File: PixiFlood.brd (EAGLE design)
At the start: 43.2 x 46 mm, 36 parts, among them IC1 WS2811-SOP8, IC2 78L05Z, T1 2N3904, T2 2N3904, T3 2N3904, U1 PT4115B89E, U2 PT4115B89E, U3 PT4115B89E, X2 22-23-2041

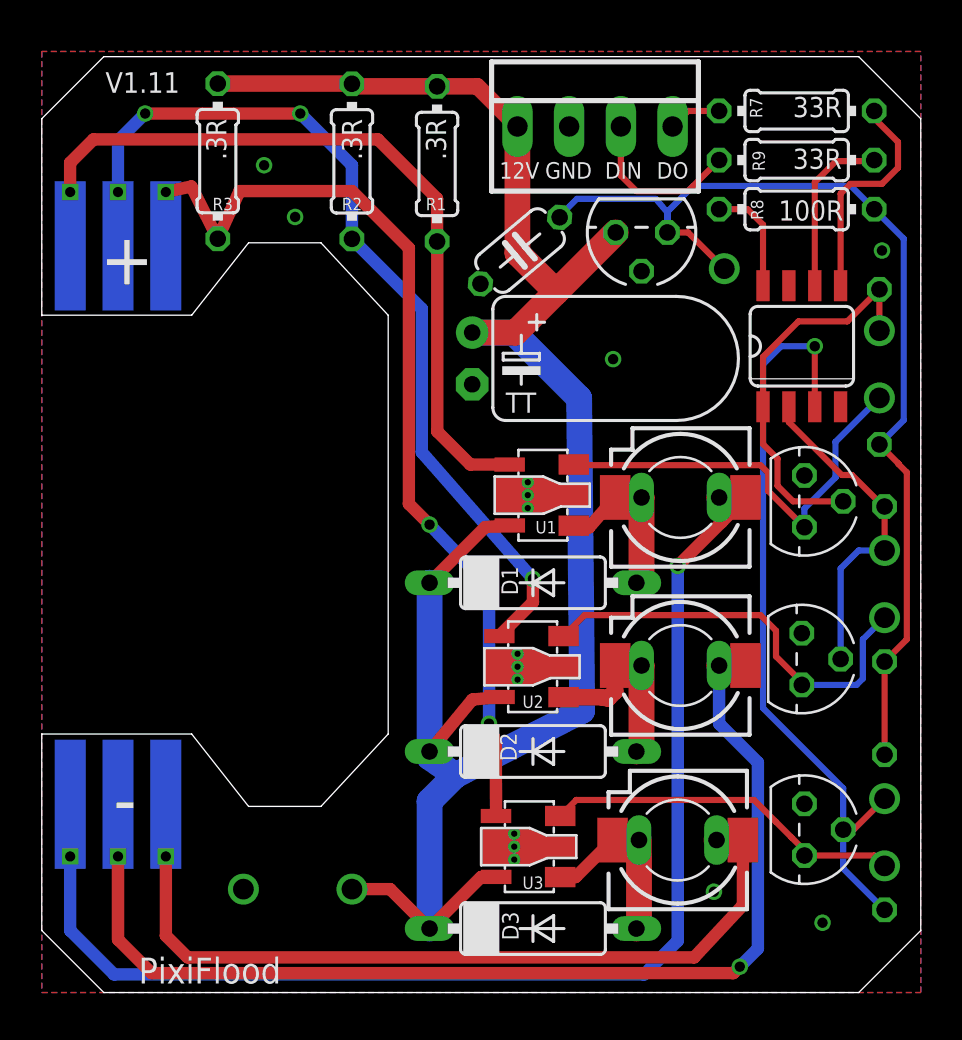
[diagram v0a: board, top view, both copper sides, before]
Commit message: Initial Commit
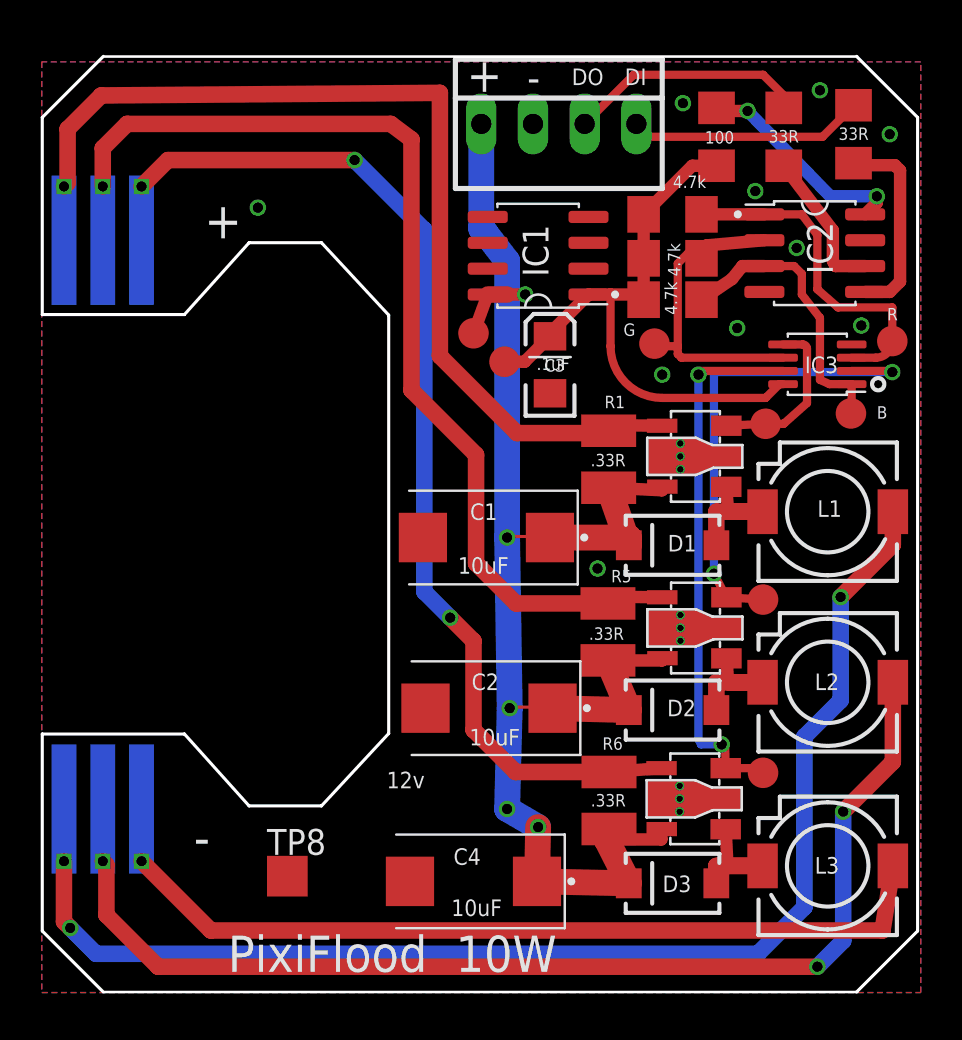
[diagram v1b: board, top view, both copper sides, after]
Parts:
- removed T$1, T$2, T$3, T$4, T$5, T$6, T$7, T$8, T$9: TEST_PINTP-2, headers:TP-2
- removed T1, T2, T3: 2N3904, transistor:TO92
- removed X2: 22-23-2041, connectors:22-23-2041
- added C3: .1uF, capacitors:EIA3216
- added C4: 10uF, capacitors:VISHAY-CASE-D
- added IC3: TC7W04FP-0.65, logic:SSOP8-0.65P-(TSSOP8)
- added TP1, TP2, TP3, TP4, TP5, TP6, TP7, TP9: TPSQTP15R, testpad:TP15R
- added TP8: TPSQTP20SQ, testpad:TP20SQ
- added X1: 22-23-2041, connectors:22-23-2041
- B1: value LED-BOARDNODIM -> LED-BOARDV4; device myBoards:LED_BOARD_V5_A -> special:LED_BOARD-V4
- C1: value 100uF -> 10uF; device rcl:TT2D6L -> capacitors:VISHAY-CASE-D
- C2: value .1uF -> 10uF; device rcl:C050-024X044 -> capacitors:VISHAY-CASE-D
- D1, D2, D3: value 1N5819 -> B340A; device diode:DO07 -> SparkFun-DiscreteSemi:SMA-DIODE
- IC1: value WS2811-SOP8 -> 78L05SMD; device MyLibrary:SO08-SKINNYPADS -> regulators:SO08
- IC2: value 78L05Z -> WS2811S; device linear:TO92 -> drivers:SO08
- L1, L2, L3: value INDUCTOR82114R -> SLF7045T-101MR60-H; device rcl:82114R-C -> inductors:SLF7045
- R1: value .3R -> .33R; device resistor:0204/7 -> resistor:R1210
- R2, R3: value .3R -> 33R; device resistor:0204/7 -> rcl:R1206
- R4: value 4.7k -> 100; device resistor:0204/7 -> rcl:R1206
- R5, R6: value 4.7k -> .33R; device resistor:0204/7 -> resistor:R1210
- R7, R9: value 33R -> 4.7k; device rcl:0204/7 -> rcl:R1206
- R8: value 100R -> 4.7k; device rcl:0204/7 -> rcl:R1206
- moved R3 31.3 mm to (39.9, 42.2)
- moved C2 22.5 mm to (22.0, 14.0), turned to 0 degrees
- moved R2 21.2 mm to (36.4, 42.0)
- moved R1 16.8 mm to (27.8, 26.2)
- moved R4 13.8 mm to (33.1, 42.0), flipped to the top
- moved R5 13.8 mm to (27.8, 17.7), flipped to the top, turned to 270 degrees
- moved IC1 13.7 mm to (24.4, 36.2), turned to 90 degrees
- moved R6 13.6 mm to (27.9, 9.43), flipped to the top
- moved R7 11.1 mm to (31.0, 34.0)
- moved C1 8.82 mm to (21.8, 22.4), turned to 0 degrees
- moved IC2 8.57 mm to (38.0, 36.3), turned to 0 degrees
- moved U3 8.46 mm to (32.1, 9.52)
- moved U2 8.22 mm to (32.1, 17.9)
- moved U1 7.73 mm to (32.1, 26.3)
- moved L3 7.47 mm to (38.6, 6.22), turned to 0 degrees
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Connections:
- removed net +12V: C1.+, D1.C, D2.C, D3.C, IC2.3, R1.1, R2.1, R3.1, T$9.P$1, U1.5, U2.5, U3.5, X2.1
- removed net DIN-R: IC1.6, R9.2
- removed net DO-R: IC1.5, R7.2
- removed net N$15: IC1.3, R6.2, T$5.P$1, T3.2
- removed net N$18: IC1.2, R5.2, T$4.P$1, T2.2
- removed net N$20: IC1.1, R4.2, T$1.P$1, T1.2
- new net BLU-WS: IC2.3, IC3.1, R7.2, TP2.TP
- new net DIN-E: R2.1, X1.3
- new net DO-E: R3.1, X1.4
- new net GREN-WS: IC2.2, IC3.6, R8.2, TP3.TP
- new net RED-WS: IC2.1, IC3.3, R9.2, TP7.TP
- new net VIN: C1.1, C2.1, C4.1, D1.C, D2.C, D3.C, IC1.8, R1.2, R5.2, R6.2, TP4.TP, U1.5, U2.5, U3.5, X1.1
- net +5V: now also C3.A, IC1.1, IC3.8, R7.1, R9.1, TP5.TP; no longer C2.1, IC2.1, R5.1, R6.1, T$2.P$1
- net BLUE: now also IC3.7, TP9.TP; no longer T$6.P$1, T3.1
- net BOUT: now also R6.1; no longer R3.2
- net DIN: now also IC2.6, R2.2; no longer R9.1, X2.3
- net DO: now also IC2.5, R3.2; no longer R7.1, X2.4
- net GND: now also C1.2, C3.C, C4.2, IC1.2, IC1.3, IC1.6, IC1.7, IC2.4, IC3.4, TP8.TP, X1.2; no longer C1.-, IC1.4, IC2.2, T$3.P$1, T1.3, T2.3, T3.3, X2.2
- net GOUT: now also R5.1; no longer R2.2
- net GREEN: now also IC3.2, TP6.TP; no longer T$7.P$1, T2.1
- net N$1: no longer L1.1@A
- net N$10: no longer L3.2@A
- net N$2: no longer L3.1@A
- net N$3: no longer L1.2@A
- net N$5: no longer L2.1@A
- net N$9: no longer L2.2@A
- net RED: now also IC3.5, TP1.TP; no longer T$8.P$1, T1.1
- net ROUT: now also R1.1; no longer R1.2
- net VDD: now also IC2.8, R4.2; no longer IC1.8, R8.2
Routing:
- net +12V: track 99.4 -> 0.00 mm
- net VIN: track 0.00 -> 78.1 mm, vias 0 -> 5
- net N$15: track 37.8 -> 0.00 mm, vias 1 -> 0
- net +5V: track 51.6 -> 29.6 mm
- net N$20: track 19.3 -> 0.00 mm
- net RED-WS: track 0.00 -> 16.9 mm
- net N$18: track 16.3 -> 0.00 mm
- net GREN-WS: track 0.00 -> 15.8 mm
- net BLU-WS: track 0.00 -> 14.3 mm
- net RED: track 21.0 -> 8.58 mm
- net DIN-E: track 0.00 -> 11.8 mm
- net DO-E: track 0.00 -> 11.6 mm
- net DO-R: track 11.1 -> 0.00 mm
- net ROUT: track 39.7 -> 50.7 mm
- net BLUE: track 17.7 -> 26.8 mm, vias 0 -> 2
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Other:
- board size 43.2 x 46 mm -> 43 x 46 mm
- board text added: "+"
- board text added: "-"
- board text added: "12v"
- board text added: "B"
- board text added: "DI"
- board text added: "G"
- board text added: "PixiFlood 10W"
- board text added: "R"
- board text added: "v2.0"
- board text removed: "12V"
- board text removed: "DIN"
- board text removed: "GND"
- board text removed: "PixiFlood"
- board text removed: "V1.11"
